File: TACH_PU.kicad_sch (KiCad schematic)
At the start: 11 parts, among them Q1 AO3400A, Q3 AO3401A

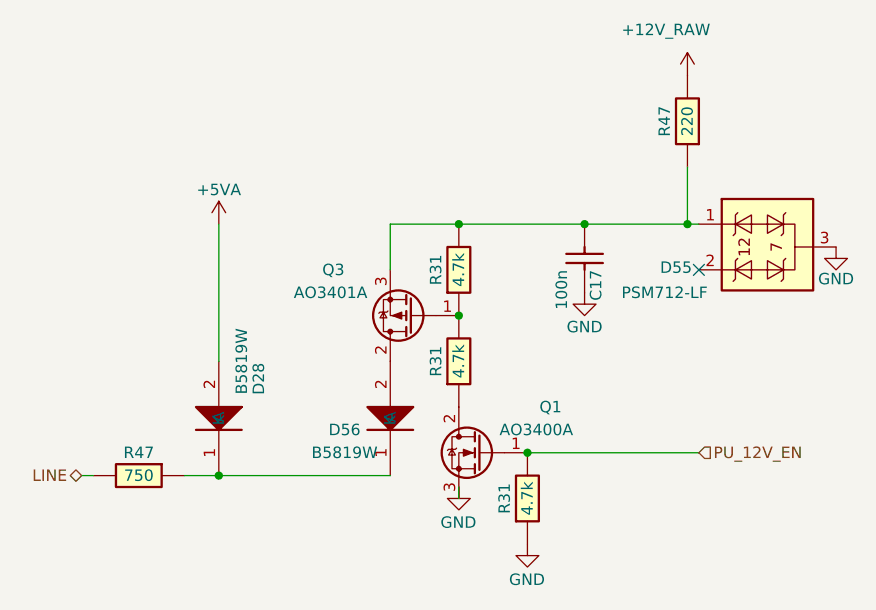
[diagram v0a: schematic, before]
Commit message: Export
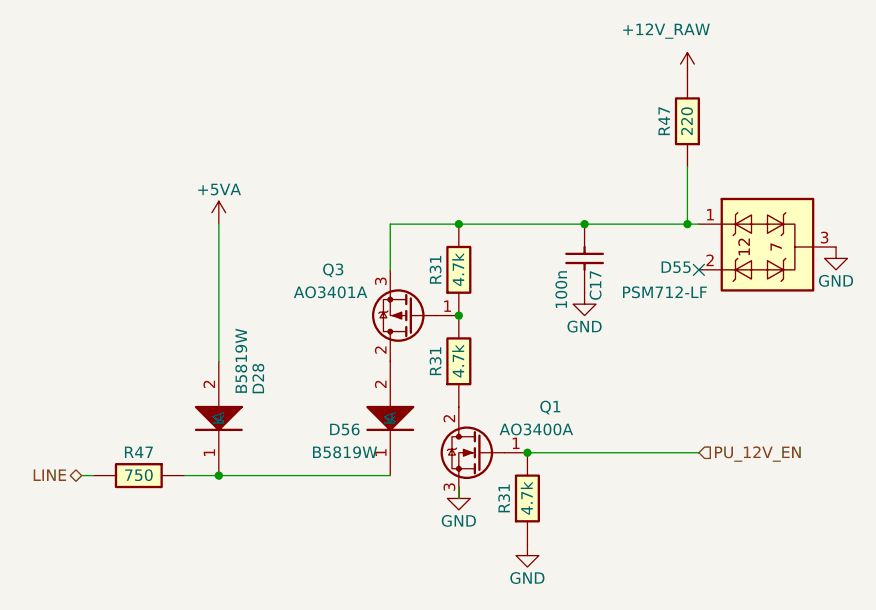
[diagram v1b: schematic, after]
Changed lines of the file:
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@@
       (effects (font (size 1.27 1.27)) hide)
     )
-    (property "Value" "GND" (at 123.1392 80.1434 0)
+    (property "Value" "GND" (at 123.19 80.01 0)
       (effects (font (size 1.27 1.27)))
     )
@@
         )
         (path "/63d2dd9f-d5ff-4811-a88d-0ba932475460/15162d4d-e221-4df0-bbe4-06499b4ace57"
-          (reference "#PWR0164") (unit 1)
+          (reference "#PWR0215") (unit 1)
         )
       )
@@
       (effects (font (size 1.27 1.27)) hide)
     )
-    (property "Value" "GND" (at 157.48 46.736 0)
+    (property "Value" "GND" (at 157.48 46.99 0)
       (effects (font (size 1.27 1.27)))
     )
@@
         )
         (path "/63d2dd9f-d5ff-4811-a88d-0ba932475460/15162d4d-e221-4df0-bbe4-06499b4ace57"
-          (reference "#PWR0166") (unit 1)
+          (reference "#PWR0213") (unit 1)
         )
       )
@@
       (effects (font (size 1.27 1.27)) hide)
     )
-    (property "Value" "GND" (at 115.5192 73.7934 0)
+    (property "Value" "GND" (at 115.57 73.66 0)
       (effects (font (size 1.27 1.27)))
     )
@@
         )
         (path "/63d2dd9f-d5ff-4811-a88d-0ba932475460/15162d4d-e221-4df0-bbe4-06499b4ace57"
-          (reference "#PWR0163") (unit 1)
+          (reference "#PWR0216") (unit 1)
         )
       )
@@
         )
         (path "/63d2dd9f-d5ff-4811-a88d-0ba932475460/15162d4d-e221-4df0-bbe4-06499b4ace57"
-          (reference "#PWR0165") (unit 1)
-        )
-      )
+          (reference "#PWR0214") (unit 1)
+        )
+      )
